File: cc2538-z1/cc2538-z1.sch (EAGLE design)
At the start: 102 parts, among them U1 CC2538, U10 DMG6602SVT, U12 SN74AVC4T774PW, U2 CC1120_RHM_32, U3 TPD2E001IDRLRQ1, U4 CP2103, U5 BSS138PS, U6 BSS138PS, U7 BSS138PS, U8 M25P16VMN6P, U9 DMG6602SVT, X1 FA-128, X2 32MHz, X3 32.768K

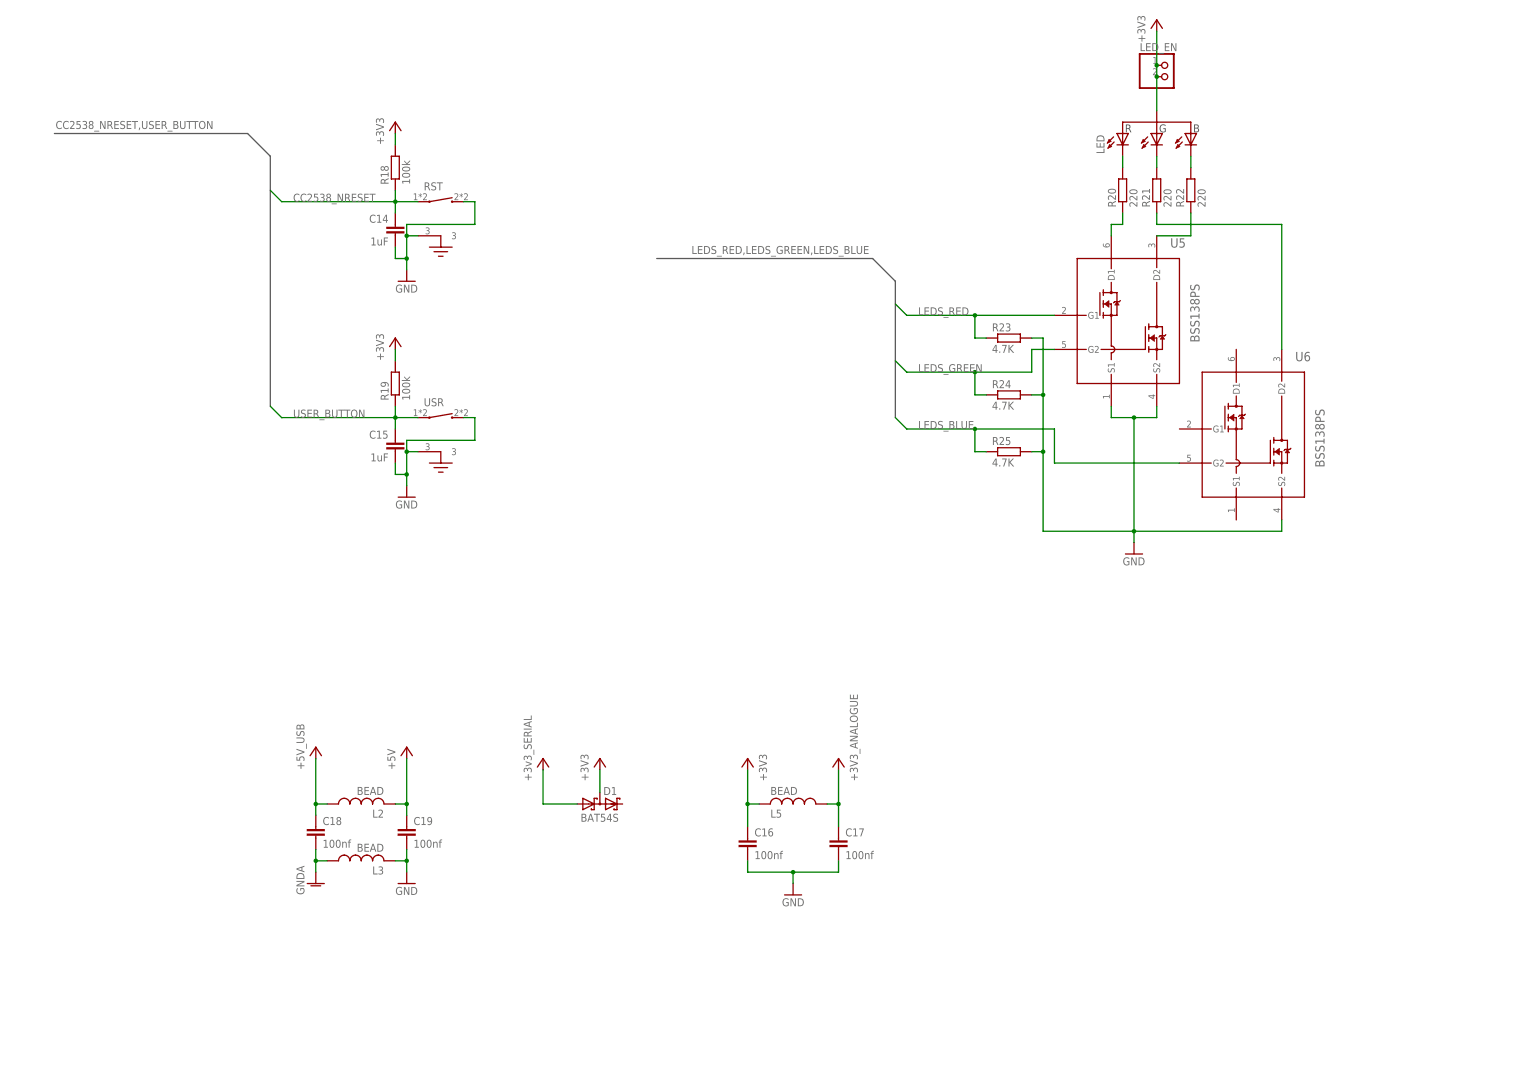
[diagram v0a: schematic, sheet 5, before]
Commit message: Finalised board design?
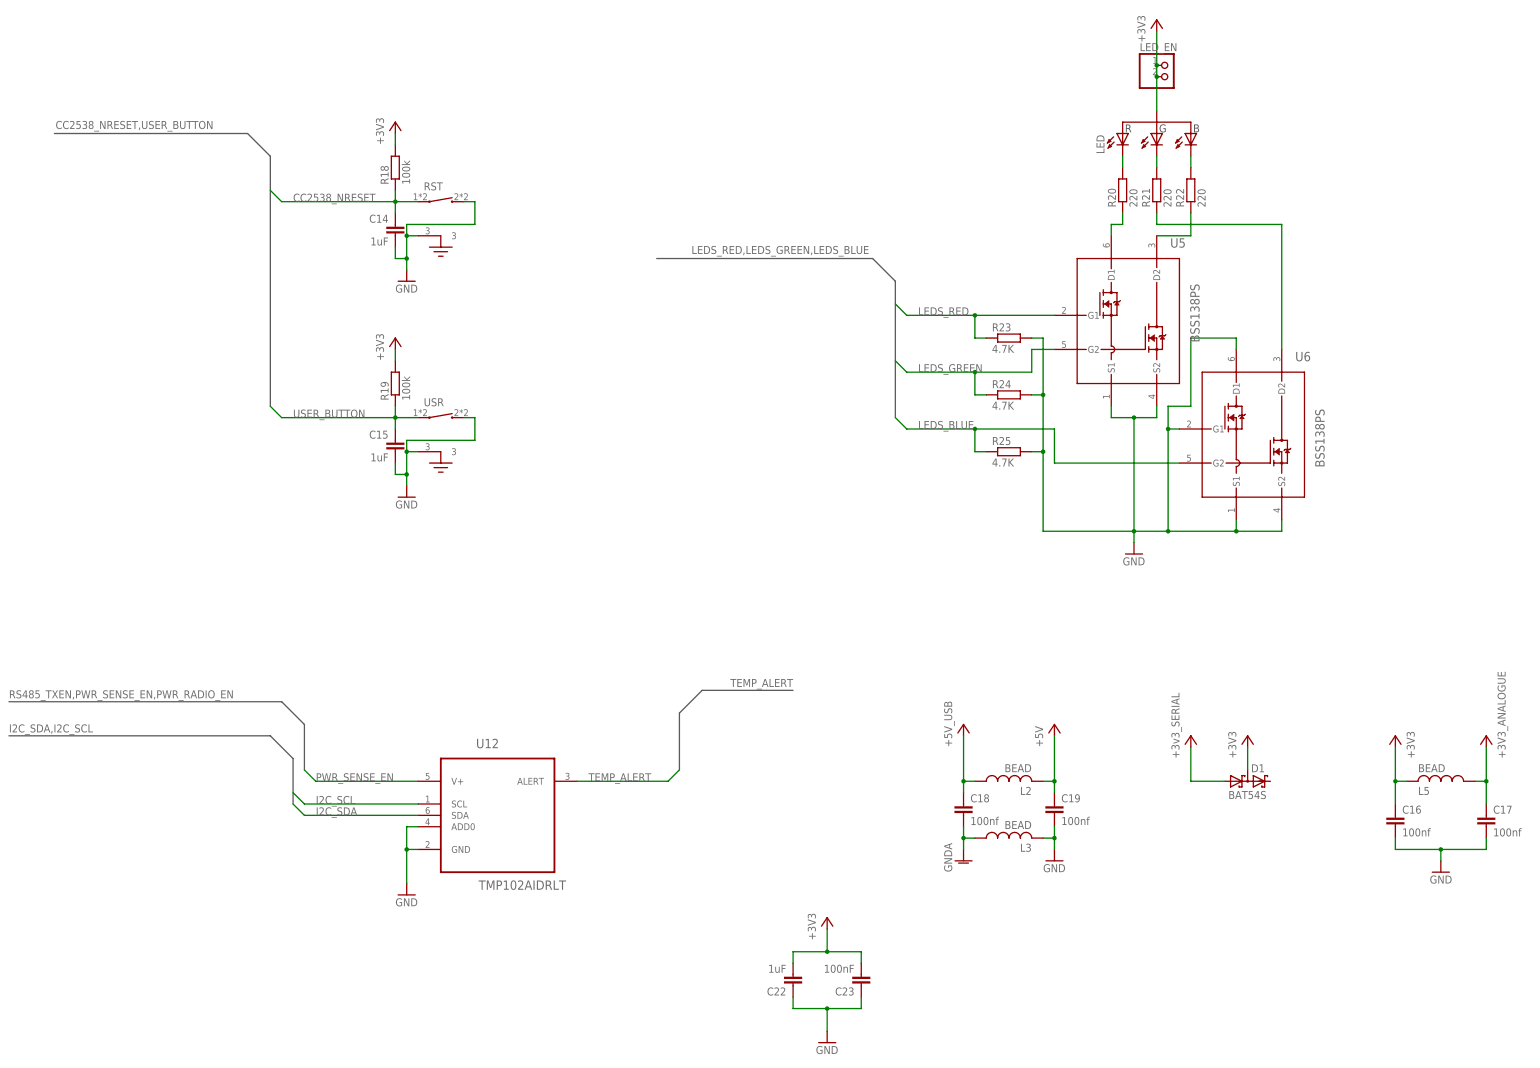
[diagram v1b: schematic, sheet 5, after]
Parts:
- added C20, C22: 1uF, CC11x:C_EUC0603S
- added C23: 100nF, CC11x:C_EUC0603S
- added U11: SN74AVC4T774PW, CC11x:SN74AVC4T774PW
- R10: value (none) -> 100k
- U12: value SN74AVC4T774PW -> TMP102AIDRLT; device CC11x:SN74AVC4T774PW -> CC11x:TMP102AIDRLT
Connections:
- removed net N$20: J1.4, R10.2
- removed net N$40: H1.ALERT
- removed net N$64: H1.TEMP_PMR
- new net TEMP_ALERT: H1.ALERT, U12.ALERT
- net +3V3: now also C22.2, C23.2, U11.DIR1, U11.DIR3, U11.DIR4, U11.VCCA; no longer U12.DIR1, U12.DIR3, U12.DIR4, U12.VCCA
- net GND: now also C20.2, C22.1, C23.1, U11.DIR2, U11.GND, U12.ADD0, U6.D1, U6.G1, U6.S1; no longer U12.DIR2
- net GNDA: no longer R10.1
- net I2C_SCL: now also U12.SCL
- net I2C_SDA: now also U12.SDA
- net JTAG_TDO/SD_PRESENCE: now also C20.1, R10.1
- net MEM_VCC: now also R10.2, U11.VCCB; no longer U12.VCCB
- net N$42: now also U11.~OE; no longer U12.~OE
- net PWR_SENSE_EN: now also H1.TEMP_PMR, U12.V+
- net SD_BUF_CLK: now also U11.B3; no longer U12.B3
- net SD_BUF_CSN: now also U11.B4; no longer U12.B4
- net SD_BUF_MISO: now also U11.B2; no longer U12.B2
- net SD_BUF_MOSI: now also U11.B1; no longer U12.B1
- net SD_SPI_CLK: now also U11.A3; no longer U12.A3
- net SD_SPI_CSN: now also U11.A4; no longer U12.A4
- net SD_SPI_MISO: now also U11.A2; no longer U12.A2
- net SD_SPI_MOSI: now also U11.A1; no longer U12.A1
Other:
- moved on the sheet: C16, C17, C18, C19, D1, L2, L3, L5
